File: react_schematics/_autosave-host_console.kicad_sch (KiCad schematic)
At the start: 8 parts, among them J3 RJ45_Shielded, U6 12-24_buck_1, U7 MAX485E

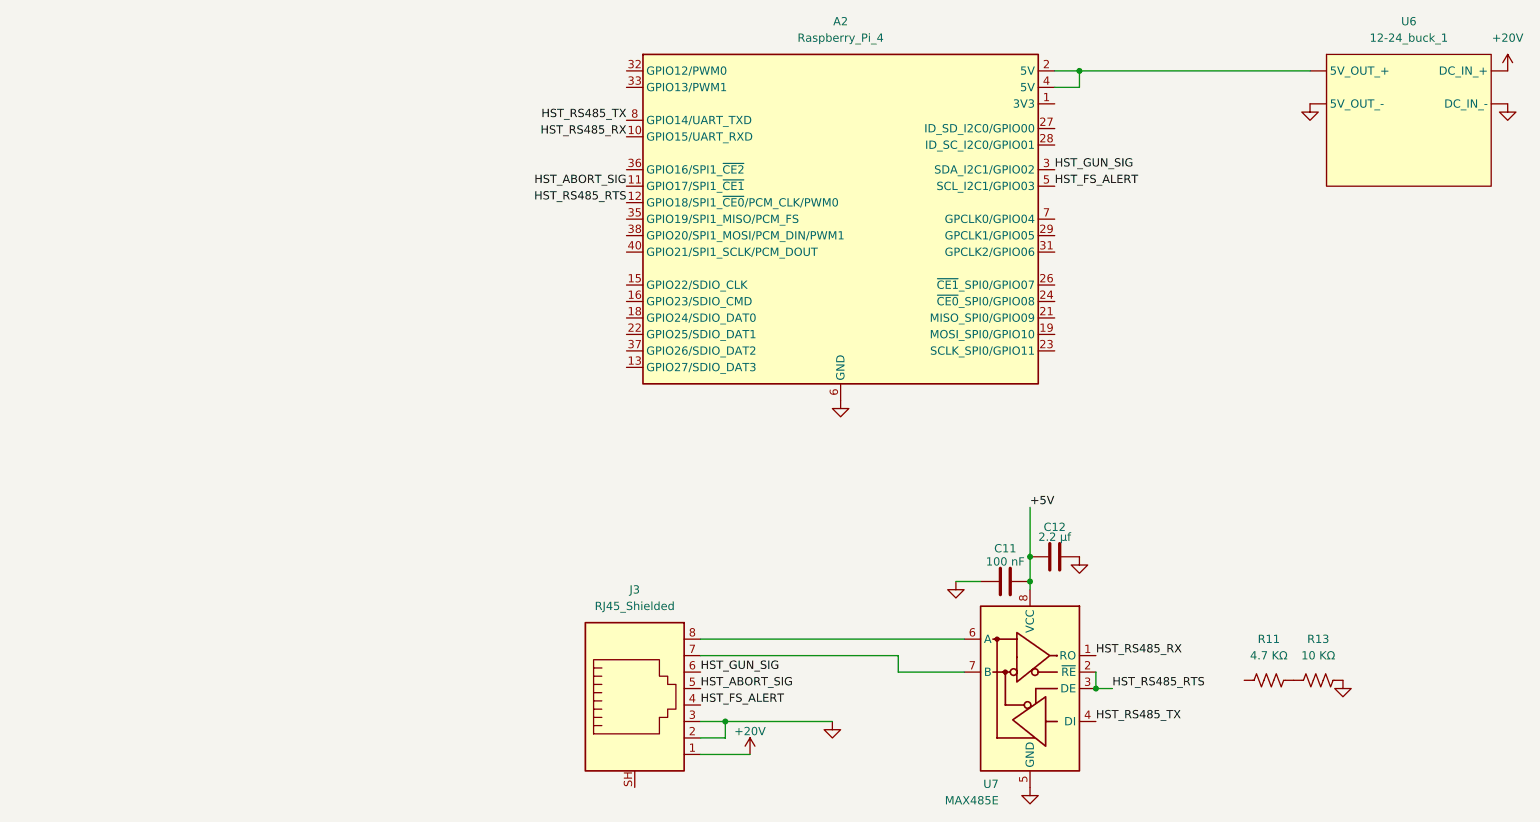
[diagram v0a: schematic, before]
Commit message: 🤪
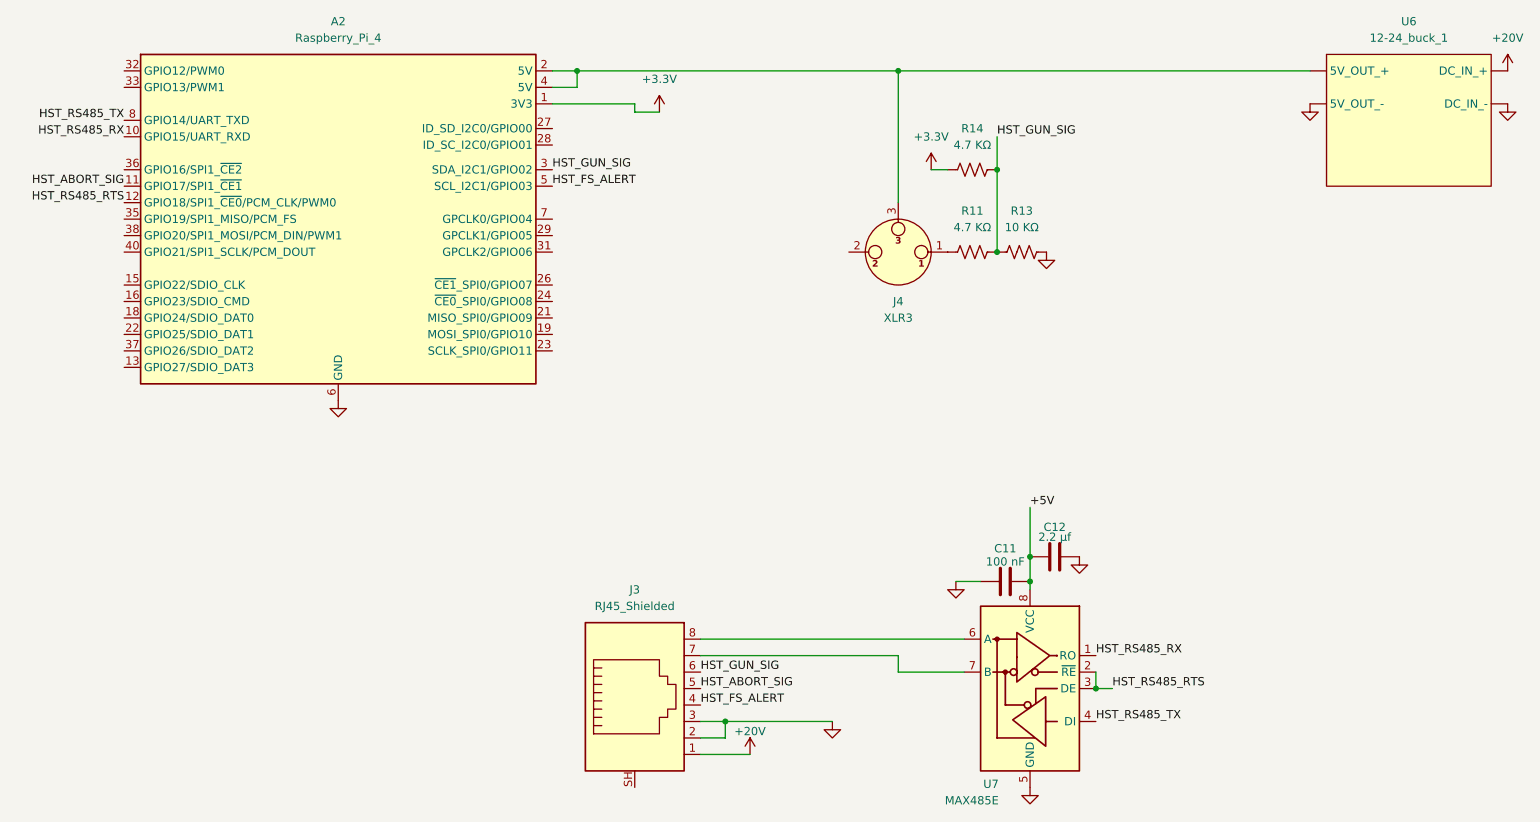
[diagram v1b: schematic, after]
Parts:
- added J4: XLR3, symbol Connector_Audio:XLR3
- added R14: 4.7 KΩ, symbol Device:R_US
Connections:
- net HST_GUN_SIG: now also R11.1, R13.2, R14.1
- net at R11.2: now also J4.1
- net +3.3V: now reaches A2.1 (3V3)
- net +3.3V: now also R14.2
- net at A2.17 (3V3), A2.2 (5V), A2.4 (5V)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: now also J4.3
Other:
- moved on the sheet: A2, R11, R13
